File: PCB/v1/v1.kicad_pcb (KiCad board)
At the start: 2 copper layers, 111 x 105 mm, 80 parts, among them J1 Screw_Terminal_01x02, Q2 BC548, SW1 Push Button, SW2 Push Button, U1 4060, U10 7400, U2 4060, U3 CD4026BE, U4 CD4026BE, U5 CD4026BE, U6 CD4026BE, U7 CD4026BE, U8 CD4026BE, Y1 32.768kHz

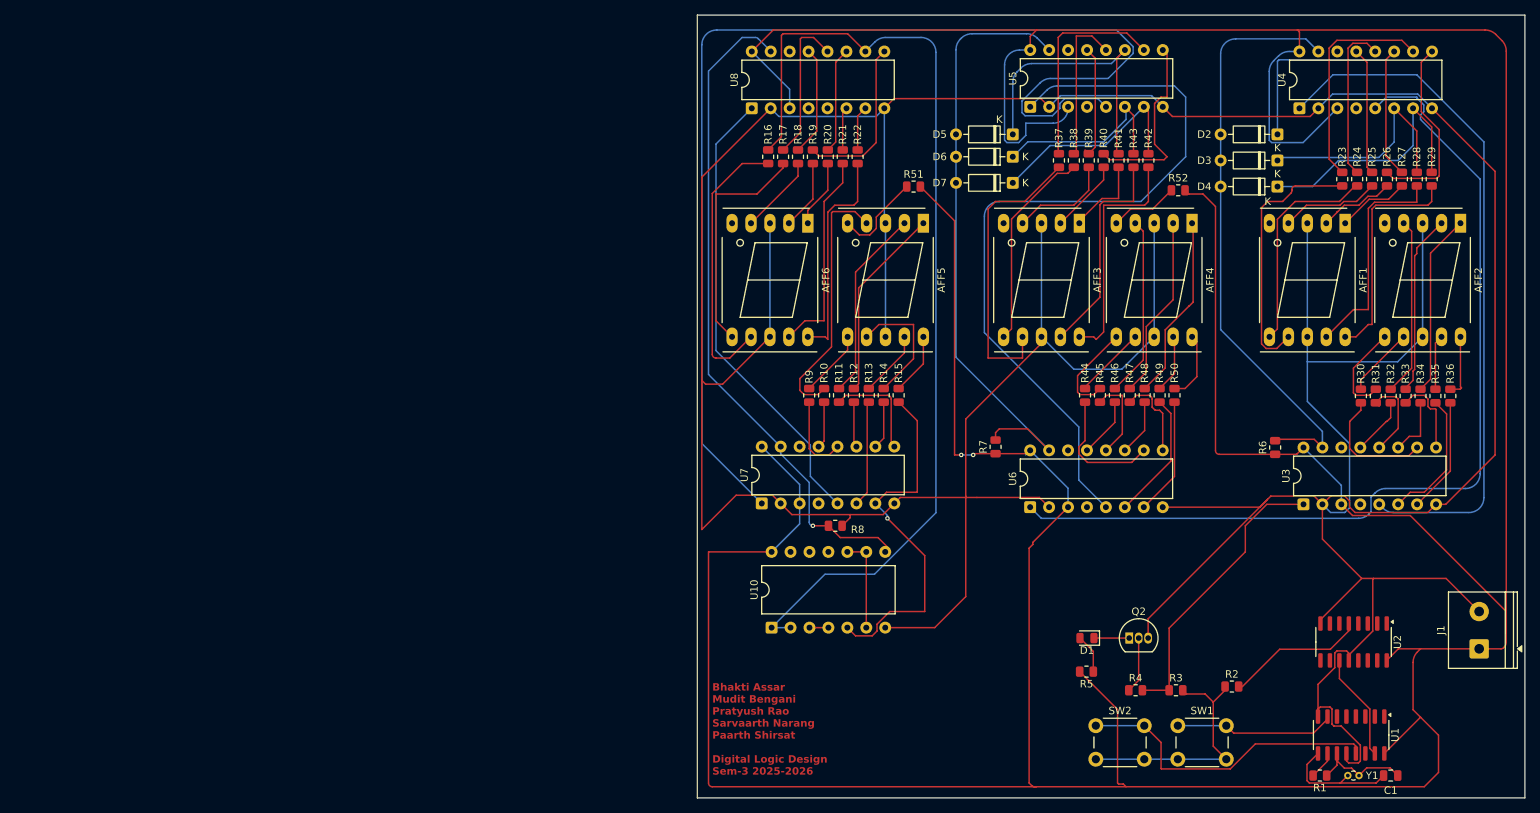
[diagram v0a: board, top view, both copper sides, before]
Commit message: Updated Schematic
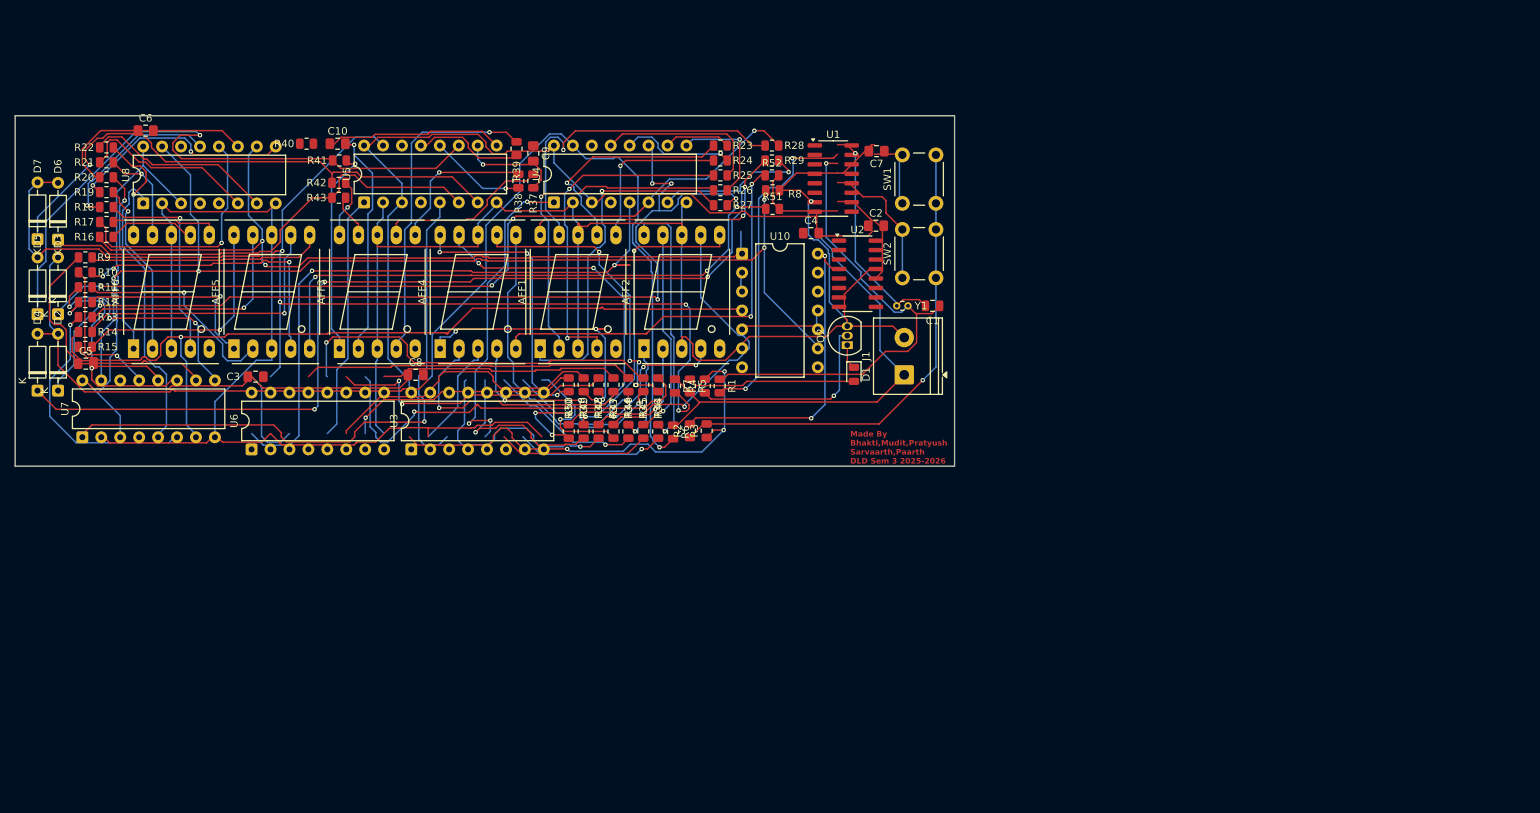
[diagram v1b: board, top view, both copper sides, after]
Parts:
- added C10: 0.1u, Capacitor_SMD:C_0805_2012Metric_Pad1.18x1.45mm_HandSolder, F.Cu at (93.8, 66.8)
- added C2: 0.1u, Capacitor_SMD:C_0805_2012Metric_Pad1.18x1.45mm_HandSolder, F.Cu at (166.0, 77.8)
- added C3: 0.1u, Capacitor_SMD:C_0805_2012Metric_Pad1.18x1.45mm_HandSolder, F.Cu at (82.8, 98.0)
- added C4: 0.1u, Capacitor_SMD:C_0805_2012Metric_Pad1.18x1.45mm_HandSolder, F.Cu at (157.2, 78.8)
- added C5: 0.1u, Capacitor_SMD:C_0805_2012Metric_Pad1.18x1.45mm_HandSolder, F.Cu at (60.0, 96.2)
- added C6: 0.1u, Capacitor_SMD:C_0805_2012Metric_Pad1.18x1.45mm_HandSolder, F.Cu at (68.0, 65.0)
- added C7: 0.1u, Capacitor_SMD:C_0805_2012Metric_Pad1.18x1.45mm_HandSolder, F.Cu at (166.0, 67.8)
- added C8: 0.1u, Capacitor_SMD:C_0805_2012Metric_Pad1.18x1.45mm_HandSolder, F.Cu at (104.2, 97.8)
- added C9: 0.1u, Capacitor_SMD:C_0805_2012Metric_Pad1.18x1.45mm_HandSolder, F.Cu at (120.0, 68.0)
- moved D4 168.5 mm to (53.5, 99.9), turned to 90 degrees
- moved D2 167.1 mm to (56.2, 99.9), turned to 90 degrees
- moved D3 164.9 mm to (56.2, 89.6), turned to 90 degrees
- moved D5 133.0 mm to (53.5, 89.6), turned to 90 degrees
- moved D7 131.0 mm to (53.5, 79.6), turned to 90 degrees
- moved D6 128.5 mm to (56.2, 79.6), turned to 90 degrees
- moved U3 119.9 mm to (103.6, 107.8)
- moved AFF2 110.8 mm to (134.8, 94.2), turned to 90 degrees
- moved R15 109.3 mm to (59.9, 94.0), turned to 180 degrees
- moved AFF1 109.3 mm to (120.9, 94.2), turned to 90 degrees
- moved R43 108.6 mm to (93.9, 72.0), turned to 0 degrees
- moved R14 107.4 mm to (59.9, 92.0), turned to 180 degrees
- moved R40 106.9 mm to (89.6, 66.8), turned to 0 degrees
- moved R42 106.7 mm to (93.9, 74.0), turned to 0 degrees
- moved R30 106.4 mm to (124.8, 105.3)
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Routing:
- net +6V: track 658.8 -> 316.9 mm, vias 2 -> 0
- net GND: track 649.5 -> 361.0 mm, vias 0 -> 1
- net Net-(D4-K): track 35.1 -> 141.5 mm, vias 0 -> 4
- net Net-(D2-A): track 80.2 -> 166.1 mm, vias 0 -> 1
- net Net-(D2-K): track 44.3 -> 129.7 mm, vias 0 -> 5
- net Net-(D3-K): track 31.1 -> 111.6 mm, vias 0 -> 4
- net Net-(D5-A): track 83.0 -> 163.2 mm, vias 0 -> 4
- net /CLK - Mod-12: track 158.5 -> 80.1 mm, vias 0 -> 1
- net Net-(U5-CLK): track 106.8 -> 33.0 mm
- net Net-(AFF5-DP): track 12.2 -> 77.1 mm, vias 0 -> 3
- net Net-(U7-G): track 49.3 -> 109.2 mm
- net Net-(U7-RESET): track 89.1 -> 145.8 mm, vias 1 -> 4
- net Net-(U3-CARRY_OUT): track 93.5 -> 42.4 mm, vias 0 -> 3
- net Net-(U1-~{Φ1}): track 14.3 -> 64.9 mm, vias 0 -> 1
- net Net-(D7-K): track 28.3 -> 74.2 mm, vias 0 -> 1
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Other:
- board size 111 x 105 mm -> 126 x 47 mm
- board text added: "Made By Bhakti,Mudit,Pratyush Sarvaarth,Paarth DLD Sem 3 2025-2026"
- board text removed: "Bhakti Assar Mudit Bengani Pratyush Rao Sarvaarth Narang Paarth Shirsat Digital Logic Design Sem-3 2025-2026"
